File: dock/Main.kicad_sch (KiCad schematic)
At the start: 67 parts, among them IC401 TLV70218_SOT23-5, IC402 USBLC6-2P6, IC403 FT230XQ, IC404 MIC5219-3.3YM5, IC405 TXB0304RUT, IC406 USBLC6-2P6, IC407 USB2512BT, IC408 USBLC6-2P6, IC409 MIC2026-1xM, J401 Jumper, J402 Voltage, Q401 BSH205G2AR, SW401 Charge, X401 Debug, X402 UART, X403 Host, X404 Device, X405 Current, Y401 24 MHz

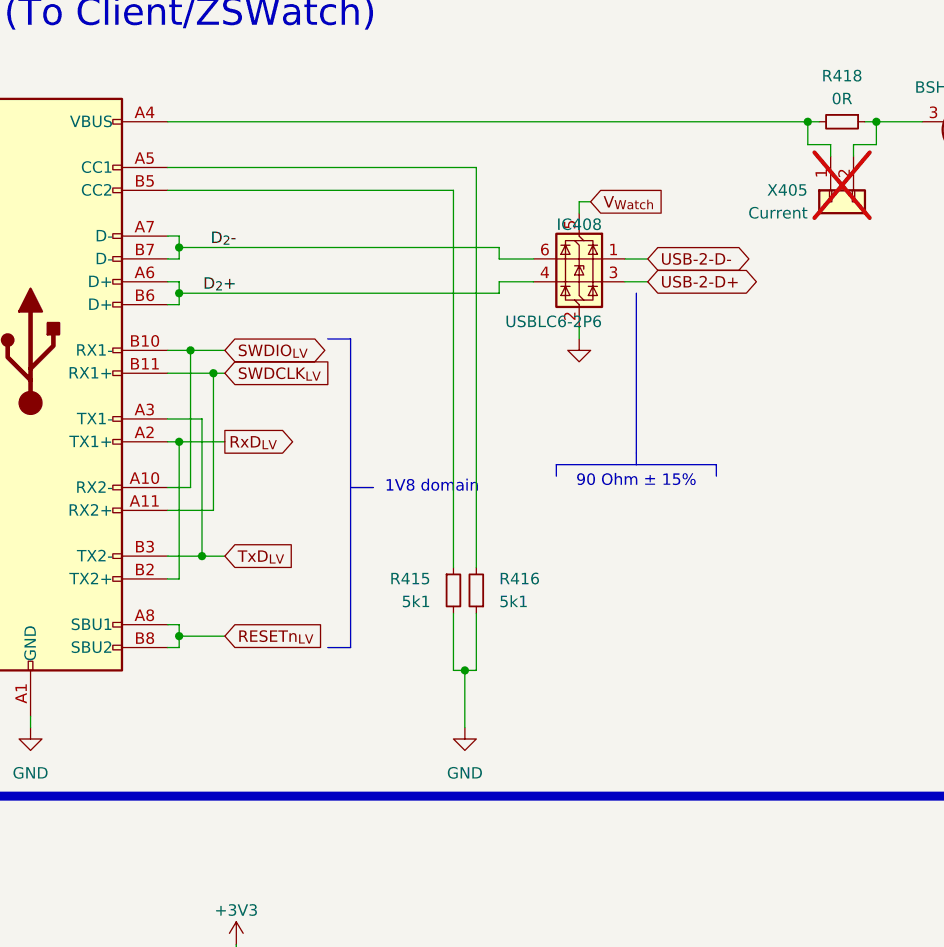
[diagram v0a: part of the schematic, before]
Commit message: Task: Issue #69
- Change ZSWatch USB to a single sided and more stable one

Closes #69

Signed-off-by: Daniel Kampert <DanielKampert@kampis-elektroecke.de>
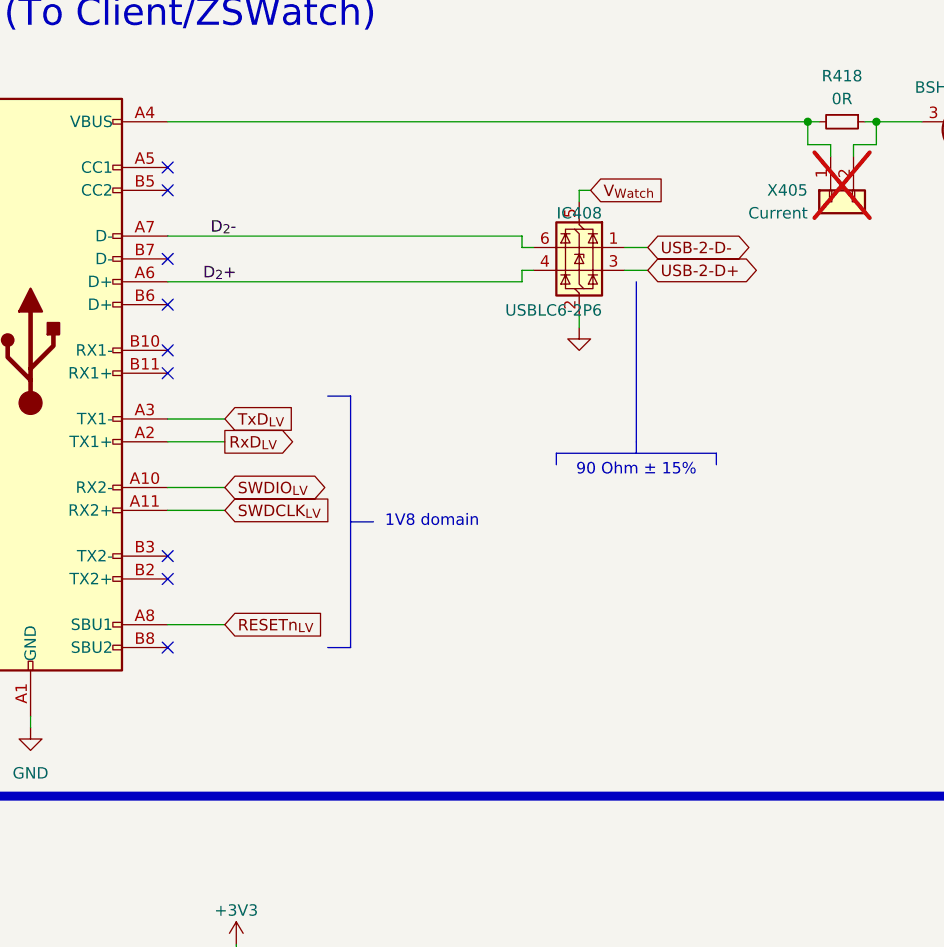
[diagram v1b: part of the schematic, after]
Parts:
- removed R415, R416: 5k1, Resistor_SMD:R_0603_1608Metric, symbol Device:R_Small
- X404: footprint Amphenol:10133475-10001LF -> GlobTect:PLUG-USBC-241SMT-4BC2SS; digikey# (none) -> 1939-PLUG-USBC-241SMT-4BC2SSCT-ND; manf Amphenol Commercial Products -> GlobTek, Inc.; manf# 10133475-10001LF -> PLUG-USBC-241SMT-4BC2SS; mouser# 523-10133475-10001LF -> (none)
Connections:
- net D_{2}+: no longer X404.B6 (D+)
- net D_{2}-: no longer X404.B7 (D-)
- net RESETn_{LV}: no longer X404.B8 (SBU2)
- net RxD_{LV}: no longer X404.B2 (TX2+)
- net SWDCLK_{LV}: no longer X404.B11 (RX1+)
- net SWDIO_{LV}: no longer X404.B10 (RX1-)
- net TxD_{LV}: no longer X404.B3 (TX2-)
- no-connect marks 23 -> 32
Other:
- moved on the sheet: IC408
